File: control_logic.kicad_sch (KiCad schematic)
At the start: 45 parts, among them SW1 KMR721NGLFS, SW2 KMR721NGLFS, U12 STM32F105RCTx, Y3 8MHz 12pF

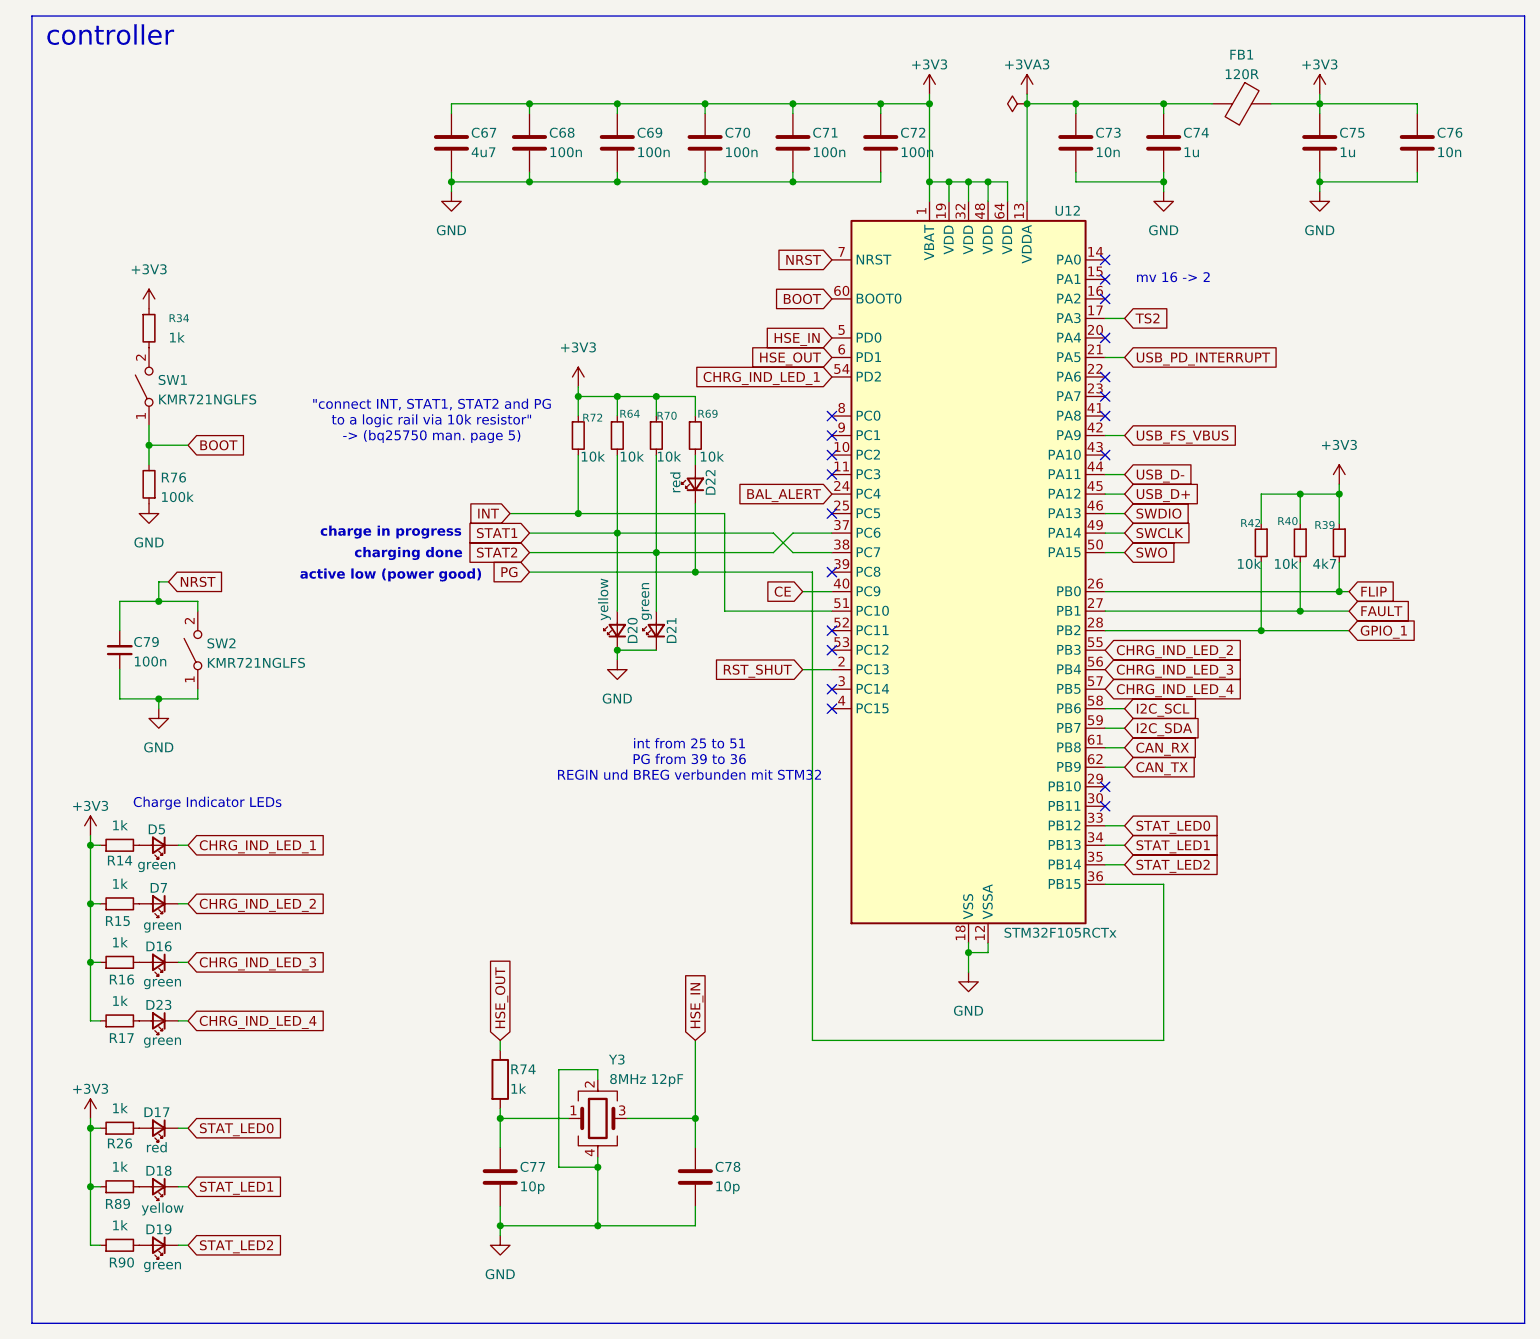
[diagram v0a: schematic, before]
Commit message: added todos
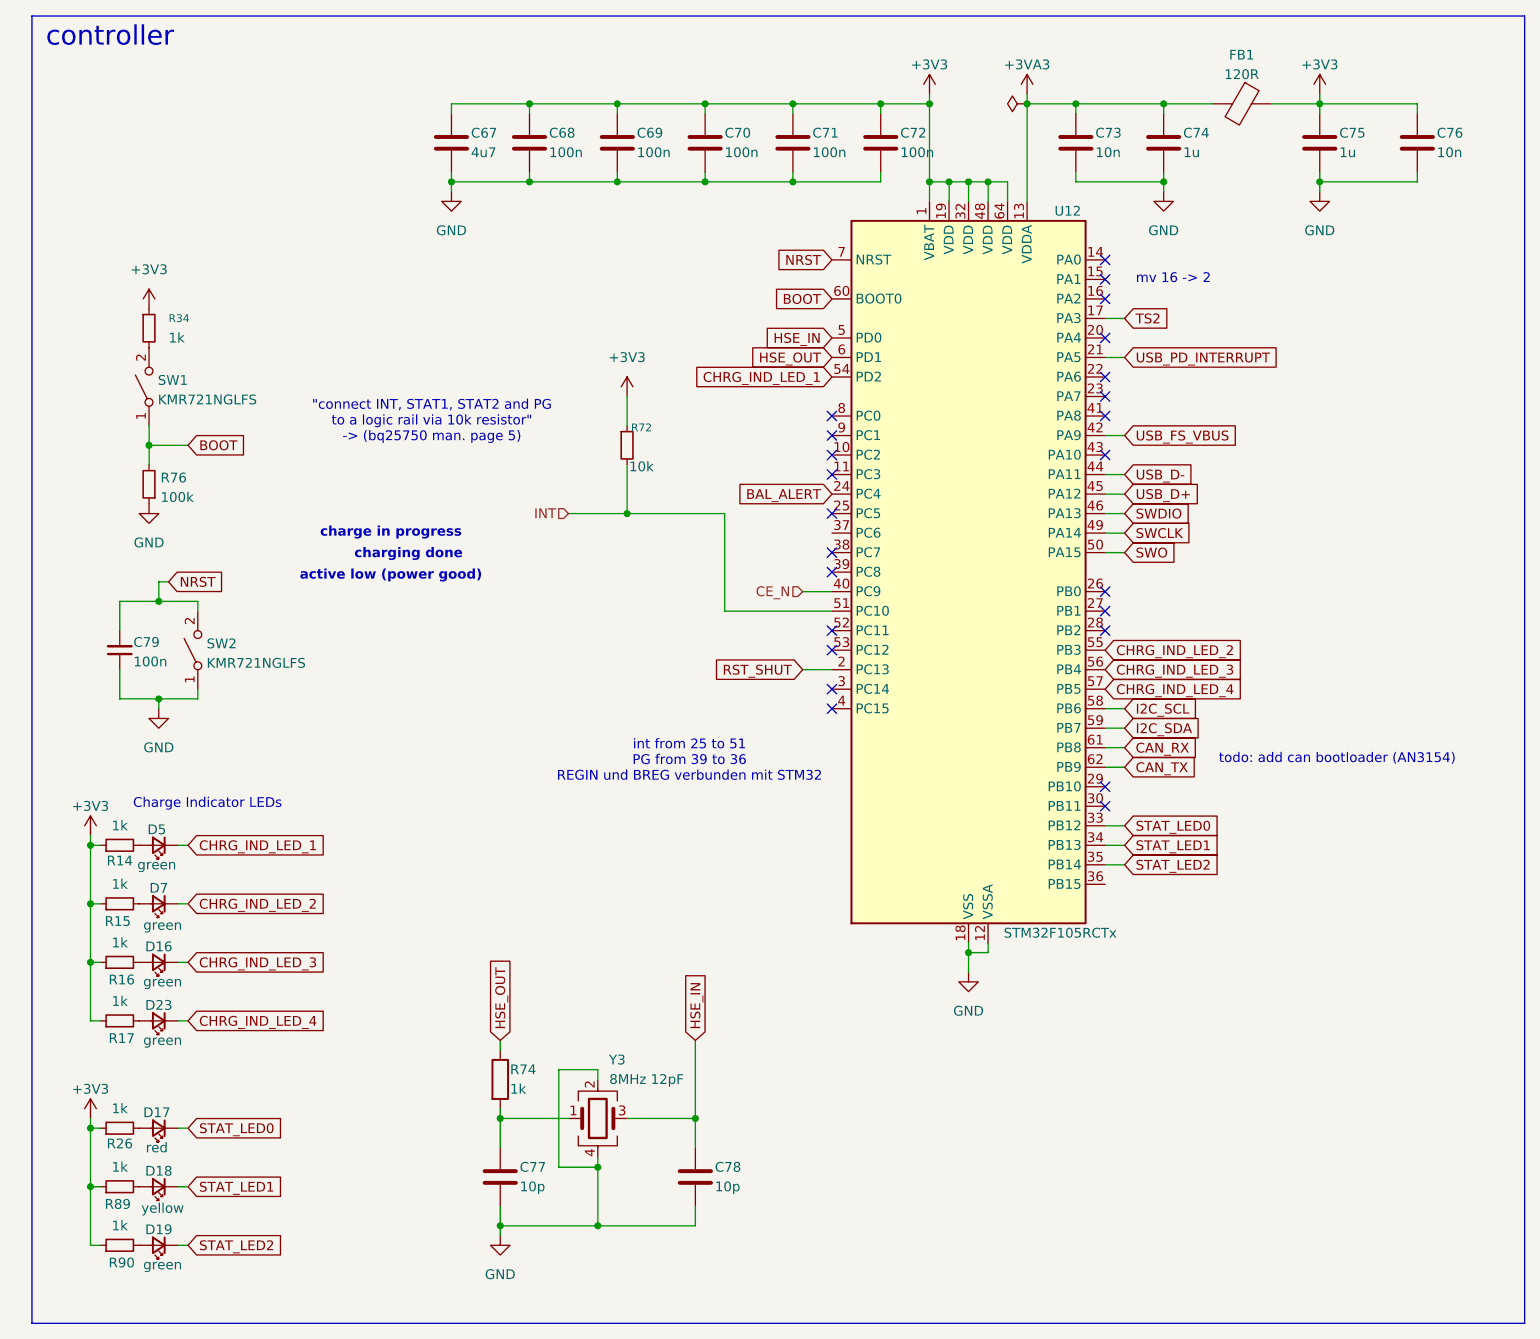
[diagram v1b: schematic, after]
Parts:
- removed D20: yellow, LED_SMD:LED_0603_1608Metric, symbol Device:LED_Small
- removed D21: green, LED_SMD:LED_0603_1608Metric, symbol Device:LED_Small
- removed D22: red, LED_SMD:LED_0603_1608Metric, symbol Device:LED_Small
- removed R39: 4k7, Resistor_SMD:R_0402_1005Metric, symbol Device:R_Small
- removed R40, R42: 10k, Resistor_SMD:R_0402_1005Metric, symbol Device:R_Small
- removed R64, R69, R70: 10k, Resistor_SMD:R_0603_1608Metric, symbol Device:R_Small
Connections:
- net CE renamed CE_N
- net FAULT: no longer names the net of U12.27 (PB1)
- net FLIP: no longer names the net of U12.26 (PB0)
- net GPIO_1: no longer names the net of U12.28 (PB2)
- net PG: no longer names the net of U12.36 (PB15)
- net STAT1: no longer names the net of U12.38 (PC7)
- net STAT2: no longer names the net of U12.37 (PC6)
- no-connect marks 20 -> 24
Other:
- note added: "todo: add can bootloader (AN3154)"
- moved on the sheet: R72
